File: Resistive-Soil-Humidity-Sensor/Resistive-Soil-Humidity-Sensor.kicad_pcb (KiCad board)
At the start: 2 copper layers, 8 parts, among them Q1 BC547, U1 L7805CV

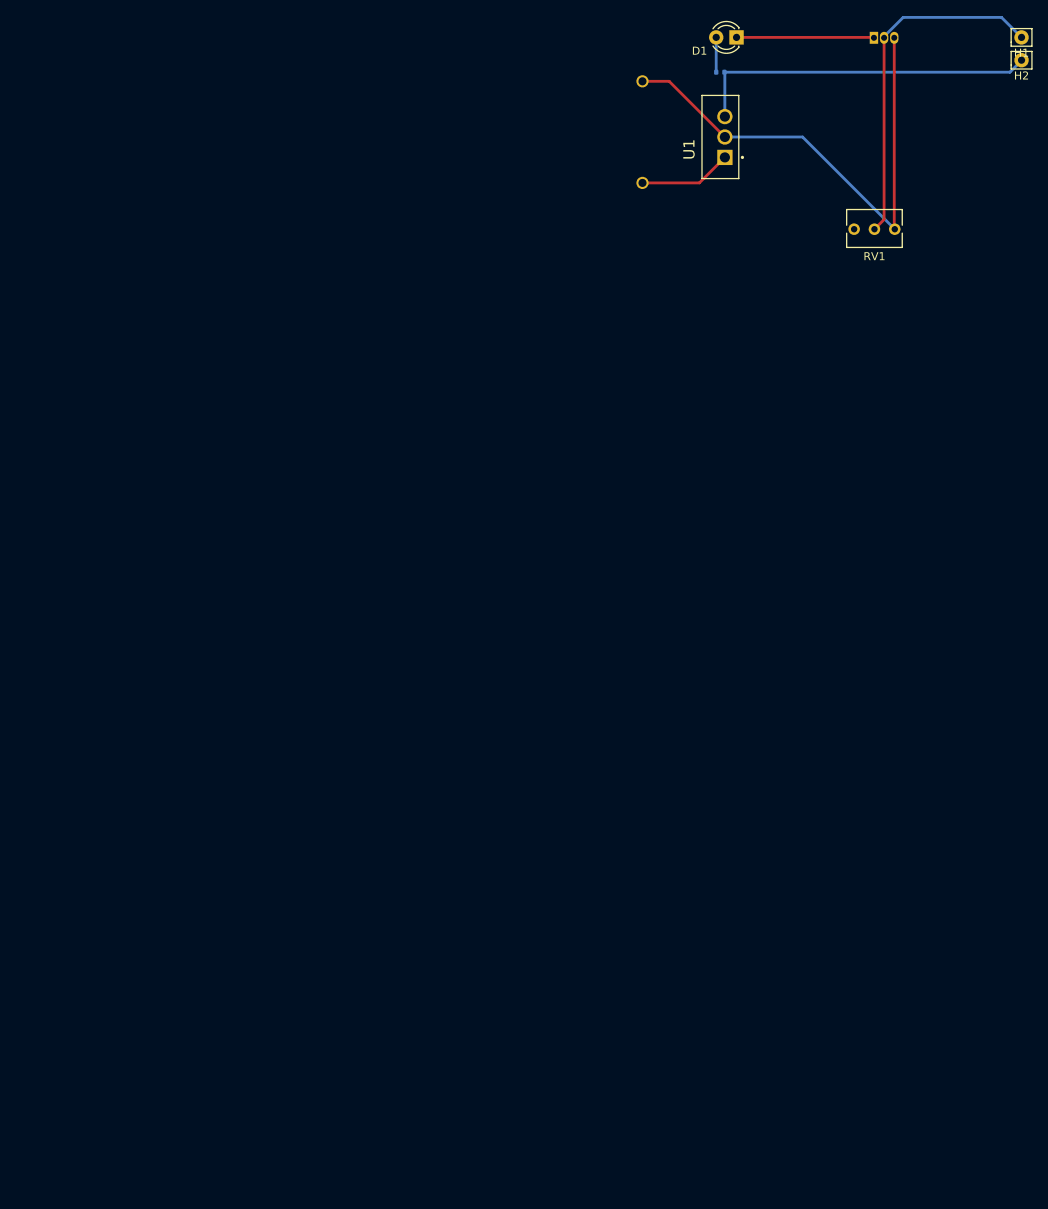
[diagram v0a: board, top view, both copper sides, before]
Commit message: update the backups
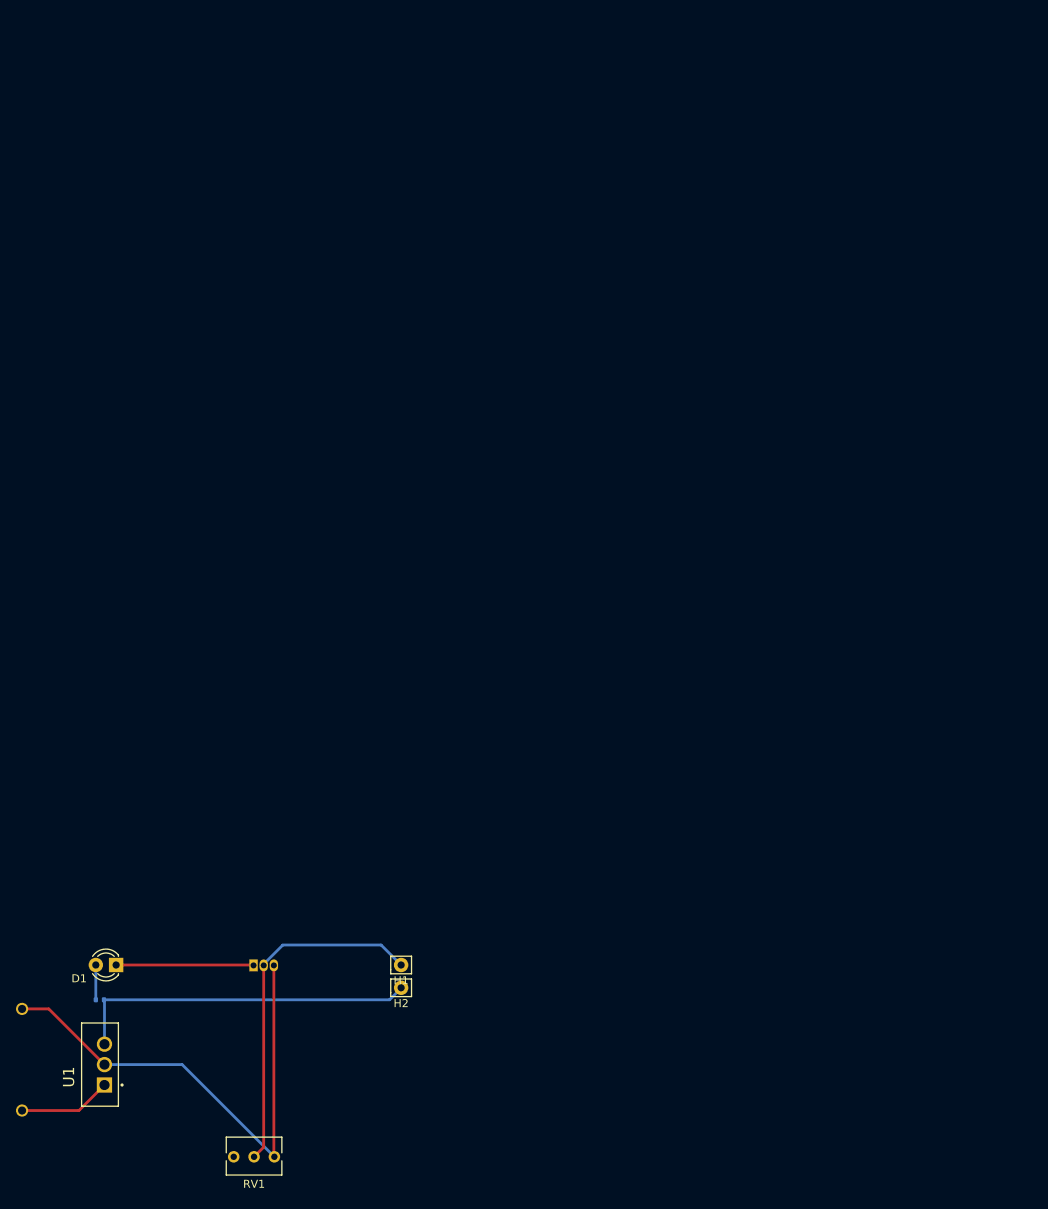
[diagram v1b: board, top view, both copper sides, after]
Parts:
- moved H2 139.5 mm to (149.7, 156.2)
- moved R1 139.5 mm to (112.0, 157.7)
- moved RV1 139.5 mm to (128.8, 177.3)
- moved 9V1 139.5 mm to (127.3, 165.2)
- moved D1 139.5 mm to (114.1, 153.3)
- moved H1 139.5 mm to (149.7, 153.3)
- moved Q1 139.5 mm to (131.2, 153.4)
- moved U1 139.5 mm to (112.6, 168.3)
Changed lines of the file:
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@@
   )
   (paper "A4")
+  (title_block
+    (comment 1 "180208063")
+  )
   (layers
     (0 "F.Cu" signal)
@@
   (net 7 "Net-(9V1-Pad+)")
   (footprint "Connector_Pin:Pin_D0.9mm_L10.0mm_W2.4mm_FlatFork" (layer "F.Cu")
-    (at 227.2415 37.3895)
+    (at 149.6915 153.3395)
     (descr "solder Pin_ with flat fork, hole diameter 0.9mm, length 10.0mm, width 2.4mm")
     (tags "solder Pin_ with flat fork")
@@
   )
   (footprint "L7805CV-Vreg:TO255P1040X460X1968-3" (layer "F.Cu")
-    (at 190.1595 52.3895 90)
+    (at 112.6095 168.3395 90)
     (property "MANUFACTURER" "STMicroelectronics")
     (property "PARTREV" "36")
@@
   )
   (footprint "Connector_Pin:Pin_D0.9mm_L10.0mm_W2.4mm_FlatFork" (layer "F.Cu")
-    (at 227.2415 40.2395)
+    (at 149.6915 156.1895)
     (descr "solder Pin_ with flat fork, hole diameter 0.9mm, length 10.0mm, width 2.4mm")
     (tags "solder Pin_ with flat fork")
@@
   )
   (footprint "LED_THT:LED_D3.0mm_FlatTop" (layer "F.Cu")
-    (at 191.6165 37.3895 180)
+    (at 114.0665 153.3395 180)
     (descr "LED, Round, FlatTop, diameter 3.0mm, 2 pins, http://www.kingbright.com/attachments/file/psearch/000/00/00/L-47XEC(Ver.9A).pdf")
     (tags "LED Round FlatTop diameter 3.0mm 2 pins")
@@
   )
   (footprint "Potentiometer_THT:Potentiometer_Bourns_3266Y_Vertical" (layer "F.Cu")
-    (at 206.3165 61.3645 180)
+    (at 128.7665 177.3145 180)
     (descr "Potentiometer, vertical, Bourns 3266Y, https://www.bourns.com/docs/Product-Datasheets/3266.pdf")
     (tags "Potentiometer vertical Bourns 3266Y")
@@
   )
   (footprint "Package_TO_SOT_THT:TO-92_Inline" (layer "B.Cu")
-    (at 208.7915 37.4395)
+    (at 131.2415 153.3895)
     (descr "TO-92 leads in-line, narrow, oval pads, drill 0.75mm (see NXP sot054_po.pdf)")
     (tags "to-92 sc-43 sc-43a sot54 PA33 transistor")
@@
   )
   (footprint "BHVPC-BatteryHolder:BAT_BH9VPC" (layer "B.Cu")
-    (at 204.8065 49.2295 180)
+    (at 127.2565 165.1795 180)
     (property "MANUFACTURER" "MPD")
     (property "MAXIMUM_PACKAGE_HEIGHT" "20.62mm")
@@
   )
   (footprint "Resistor_SMD:R_0402_1005Metric" (layer "B.Cu")
-    (at 189.5915 41.7395 180)
+    (at 112.0415 157.6895 180)
     (descr "Resistor SMD 0402 (1005 Metric), square (rectangular) end terminal, IPC_7351 nominal, (Body size source: IPC-SM-782 page 72, https://www.pcb-3d.com/wordpress/wp-content/uploads/ipc-sm-782a_amendment_1_and_2.pdf), generated with kicad-footprint-generator")
     (tags "resistor")
@@
   )
   (dimension (type aligned) (layer "B.Cu")
-    (pts (xy 177.4915 64.4895) (xy 232.2915 64.5895))
+    (pts (xy 99.9415 180.4395) (xy 154.7415 180.5395))
     (height 4.500904)
-    (gr_text "54,8001 mm" (at 204.886572 67.2404 359.8954458) (layer "B.Cu")
+    (gr_text "54,8001 mm" (at 127.336572 183.1904 359.8954458) (layer "B.Cu")
       (effects (font (size 1.5 1.5) (thickness 0.3)))
     )
@@
   )
   (dimension (type aligned) (layer "B.Cu")
-    (pts (xy 177.3815 33.9795) (xy 177.3815 64.4795))
+    (pts (xy 99.8315 149.9295) (xy 99.8315 180.4295))
     (height 4.44)
-    (gr_text "30,5000 mm" (at 171.1415 49.2295 90) (layer "B.Cu")
+    (gr_text "30,5000 mm" (at 93.5915 165.1795 90) (layer "B.Cu")
       (effects (font (size 1.5 1.5) (thickness 0.3)))
     )
@@
     (style (thickness 0.1) (arrow_length 1.27) (text_position_mode 0) (extension_height 0.58642) (extension_offset 0.5) keep_text_aligned)
   )
-  (segment (start 210.0615 37.4395) (end 210.0615 60.1595) (width 0.35) (layer "F.Cu") (net 2))
-  (segment (start 210.0615 60.1595) (end 208.8565 61.3645) (width 0.35) (layer "F.Cu") (net 2))
-  (segment (start 212.4415 34.8895) (end 224.7415 34.8895) (width 0.35) (layer "B.Cu") (net 2))
-  (segment (start 224.7415 34.8895) (end 227.2415 37.3895) (width 0.35) (layer "B.Cu") (net 2))
-  (segment (start 210.0615 37.282418) (end 212.4415 34.902418) (width 0.35) (layer "B.Cu") (net 2))
-  (segment (start 212.4415 34.902418) (end 212.4415 34.8895) (width 0.25) (layer "B.Cu") (net 2))
-  (segment (start 210.0615 37.4395) (end 210.0615 37.282418) (width 0.25) (layer "B.Cu") (net 2))
-  (segment (start 191.6165 37.3895) (end 208.7415 37.3895) (width 0.35) (layer "F.Cu") (net 3))
-  (segment (start 208.7415 37.3895) (end 208.7915 37.4395) (width 0.25) (layer "F.Cu") (net 3))
-  (segment (start 189.0765 41.7345) (end 189.0765 37.3895) (width 0.35) (layer "B.Cu") (net 4))
-  (segment (start 189.0815 41.7395) (end 189.0765 41.7345) (width 0.25) (layer "B.Cu") (net 4))
-  (segment (start 190.1595 41.7975) (end 190.1015 41.7395) (width 0.25) (layer "B.Cu") (net 5))
-  (segment (start 190.1015 41.7395) (end 225.7915 41.7395) (width 0.35) (layer "B.Cu") (net 5))
-  (segment (start 190.1595 47.2895) (end 190.1595 41.7975) (width 0.35) (layer "B.Cu") (net 5))
-  (segment (start 225.7915 41.7395) (end 227.2915 40.2395) (width 0.35) (layer "B.Cu") (net 5))
-  (segment (start 179.8615 42.8795) (end 183.1995 42.8795) (width 0.35) (layer "F.Cu") (net 6))
-  (segment (start 183.1995 42.8795) (end 190.1595 49.8395) (width 0.35) (layer "F.Cu") (net 6))
-  (segment (start 211.3315 37.4395) (end 211.3315 61.2995) (width 0.35) (layer "F.Cu") (net 6))
-  (segment (start 211.3315 61.2995) (end 211.3965 61.3645) (width 0.25) (layer "F.Cu") (net 6))
-  (segment (start 199.8715 49.8395) (end 211.3965 61.3645) (width 0.35) (layer "B.Cu") (net 6))
-  (segment (start 190.1595 49.8395) (end 199.8715 49.8395) (width 0.35) (layer "B.Cu") (net 6))
-  (segment (start 186.9695 55.5795) (end 190.1595 52.3895) (width 0.35) (layer "F.Cu") (net 7))
-  (segment (start 179.8615 55.5795) (end 186.9695 55.5795) (width 0.35) (layer "F.Cu") (net 7))
+  (segment (start 132.5115 153.3895) (end 132.5115 176.1095) (width 0.35) (layer "F.Cu") (net 2))
+  (segment (start 132.5115 176.1095) (end 131.3065 177.3145) (width 0.35) (layer "F.Cu") (net 2))
+  (segment (start 134.8915 150.8395) (end 147.1915 150.8395) (width 0.35) (layer "B.Cu") (net 2))
+  (segment (start 147.1915 150.8395) (end 149.6915 153.3395) (width 0.35) (layer "B.Cu") (net 2))
+  (segment (start 132.5115 153.232418) (end 134.8915 150.852418) (width 0.35) (layer "B.Cu") (net 2))
+  (segment (start 134.8915 150.852418) (end 134.8915 150.8395) (width 0.25) (layer "B.Cu") (net 2))
+  (segment (start 132.5115 153.3895) (end 132.5115 153.232418) (width 0.25) (layer "B.Cu") (net 2))
+  (segment (start 114.0665 153.3395) (end 131.1915 153.3395) (width 0.35) (layer "F.Cu") (net 3))
+  (segment (start 131.1915 153.3395) (end 131.2415 153.3895) (width 0.25) (layer "F.Cu") (net 3))
+  (segment (start 111.5265 157.6845) (end 111.5265 153.3395) (width 0.35) (layer "B.Cu") (net 4))
+  (segment (start 111.5315 157.6895) (end 111.5265 157.6845) (width 0.25) (layer "B.Cu") (net 4))
+  (segment (start 112.6095 157.7475) (end 112.5515 157.6895) (width 0.25) (layer "B.Cu") (net 5))
+  (segment (start 112.5515 157.6895) (end 148.2415 157.6895) (width 0.35) (layer "B.Cu") (net 5))
+  (segment (start 112.6095 163.2395) (end 112.6095 157.7475) (width 0.35) (layer "B.Cu") (net 5))
+  (segment (start 148.2415 157.6895) (end 149.7415 156.1895) (width 0.35) (layer "B.Cu") (net 5))
+  (segment (start 102.3115 158.8295) (end 105.6495 158.8295) (width 0.35) (layer "F.Cu") (net 6))
+  (segment (start 105.6495 158.8295) (end 112.6095 165.7895) (width 0.35) (layer "F.Cu") (net 6))
+  (segment (start 133.7815 153.3895) (end 133.7815 177.2495) (width 0.35) (layer "F.Cu") (net 6))
+  (segment (start 133.7815 177.2495) (end 133.8465 177.3145) (width 0.25) (layer "F.Cu") (net 6))
+  (segment (start 122.3215 165.7895) (end 133.8465 177.3145) (width 0.35) (layer "B.Cu") (net 6))
+  (segment (start 112.6095 165.7895) (end 122.3215 165.7895) (width 0.35) (layer "B.Cu") (net 6))
+  (segment (start 109.4195 171.5295) (end 112.6095 168.3395) (width 0.35) (layer "F.Cu") (net 7))
+  (segment (start 102.3115 171.5295) (end 109.4195 171.5295) (width 0.35) (layer "F.Cu") (net 7))
 )
